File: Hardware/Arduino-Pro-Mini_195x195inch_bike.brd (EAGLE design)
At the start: 49.5 x 49.5 mm, 31 parts, among them Q1 8/16/20MHz, U1 ATMEGA328, U2 MIC5205

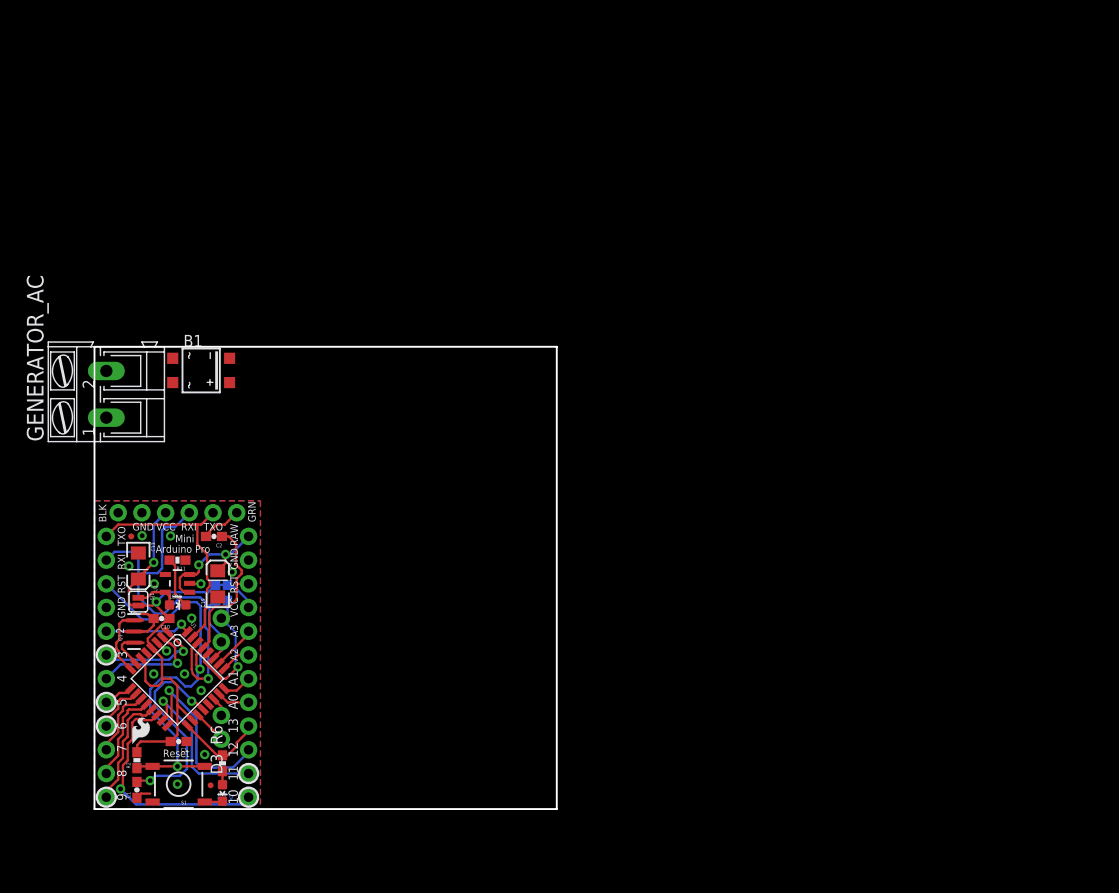
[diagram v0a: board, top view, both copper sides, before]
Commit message: work update, bike draft
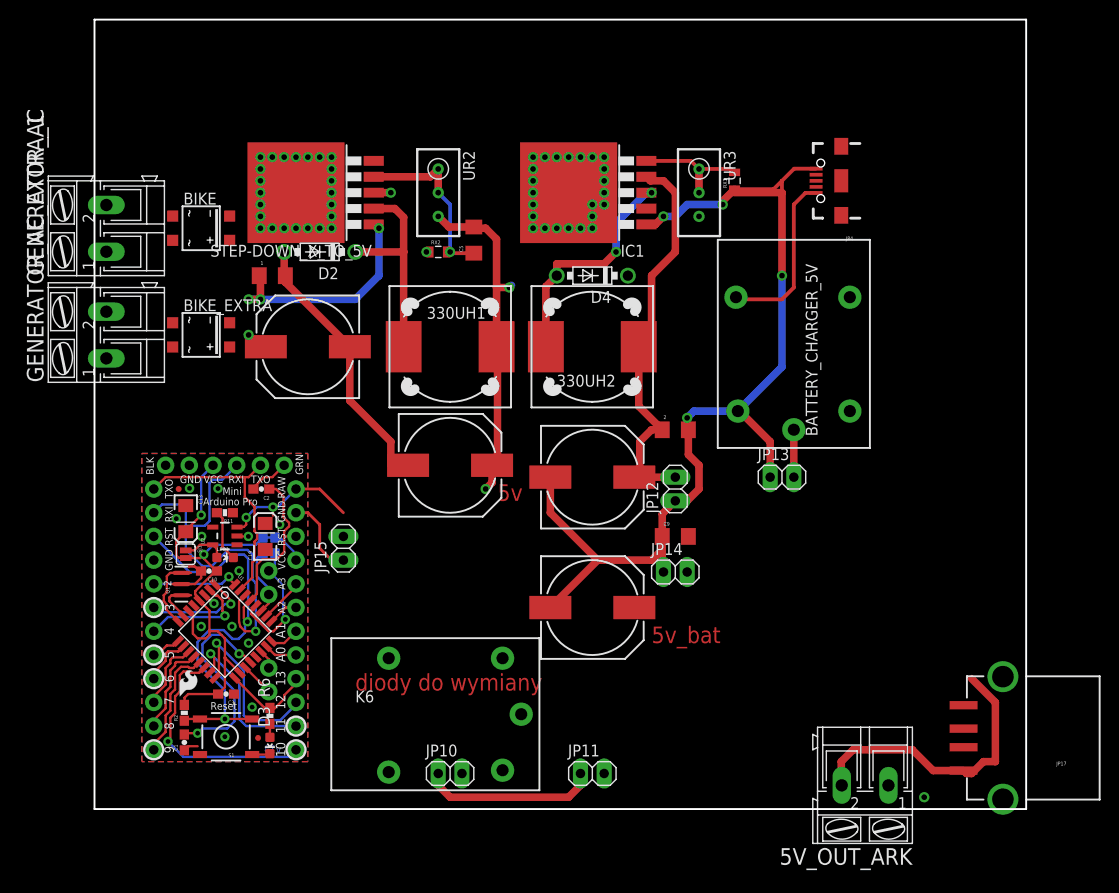
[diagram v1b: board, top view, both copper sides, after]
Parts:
- removed B1: MB1S, rectifier:SOIC-4
- added 1, 2, C5, C9: 100nF, SparkFun-Capacitors:1206
- added 330UH1, 330UH2: DR125, inductors:DR125
- added 5V_OUT_ARK, GENERATOR_AC_EXTRA_1: (no value), con-ptr500:AK300/2
- added BATTERY_CHARGER_5V, K6: ZNS5106, relay:ZN5
- added BIKE, BIKE_EXTRA: MB1S, rectifier:SOIC-4
- added C4, C6, C7, C8: 220uF, SparkFun-Capacitors:NIC_10X10.5_CAP
- added D2, D4: 1N5819-B, diode:DO41-7.6
- added IC1: XL6009_FROM_LM2596S, xl6009:TO263-5
- added JP10, JP11, JP12, JP13, JP14, JP15: (no value), pinhead:1X02
- added JP17: USB_, SparkFun-Connectors:USB-A-S-SILK-FEMALE
- added JP4: USB_MICROB_PLUGCONN-11752, SparkFun-Connectors:USB-B-MICRO-SMD_V03
- added RX2, RX3: 330R, SparkFun-Passives:0805
- added STEP-DOWN_X_TO_5V: LM2596S, national-semiconductor:TO263-5
- added UR2, UR3: 10k, rcl:RTRIM3296W
- moved GENERATOR_AC 17.8 mm to (1.27, 62.2)
- moved C19 7.18 mm to (18.3, 29.2)
- moved LED1 7.18 mm to (14.0, 26.9)
- moved Q1 7.18 mm to (9.32, 24.1)
- moved R1 7.18 mm to (18.1, 28.2)
- moved R3 7.18 mm to (19.3, 28.2)
- moved U$3 7.18 mm to (17.7, 31.5)
- moved C1 7.18 mm to (9.63, 7.14)
- moved C3 7.18 mm to (14.1, 12.3)
- moved D3 7.18 mm to (18.8, 6.81)
- moved JP3 7.18 mm to (18.7, 12.6)
- moved JP7 7.18 mm to (6.35, 6.35)
- moved JP8 7.18 mm to (17.5, 7.62)
- moved R2 7.18 mm to (9.63, 10.3)
- moved R6 7.18 mm to (18.8, 9.98)
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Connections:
- new net 3-4V_LI-ION: 2.1, 330UH2.1, C7.+, IC1.4, JP12.2
- new net 5V: 330UH1.2, BATTERY_CHARGER_5V.12, C5.2, C6.+, JP10.2, JP4.VBUS1, K6.14, UR2.3
- new net 5V_FROM_BATTERY: C19.A, C8.+, C9.2, D4.C, JP14.2, JP15.2, K6.12, U2.1, U2.3, UR3.3
- new net BIKE: BIKE.~2, GENERATOR_AC.1
- new net BIKE+: 1.1, BIKE.+, BIKE_EXTRA.+, C4.+, STEP-DOWN_X_TO_5V.1
- new net N$15: C5.1, RX2.2, STEP-DOWN_X_TO_5V.4, UR2.1, UR2.2
- new net N$16: BATTERY_CHARGER_5V.11, JP13.2
- new net N$17: 330UH1.1, D2.C, STEP-DOWN_X_TO_5V.2
- new net N$19: IC1.5, RX3.2, UR3.1, UR3.2
- new net N$21: 5V_OUT_ARK.2, JP11.2, JP17.VBUS, K6.11
- new net N$25: K6.A1
- new net N$26: BATTERY_CHARGER_5V.A1
- new net N$8: BIKE_EXTRA.~2, GENERATOR_AC_EXTRA_1.1
- new net N$9: BIKE_EXTRA.~1, GENERATOR_AC_EXTRA_1.2
- net GND: now also 1.2, 2.2, 5V_OUT_ARK.1, BATTERY_CHARGER_5V.A2, BIKE.-, BIKE_EXTRA.-, C4.-, C6.-, C7.-, C8.-, C9.1, D2.A, IC1.1, JP10.1, JP11.1, JP12.1, JP13.1, JP14.1, JP15.1, JP17.GND, JP4.GND1, K6.A2, RX2.1, RX3.1, STEP-DOWN_X_TO_5V.3, STEP-DOWN_X_TO_5V.5
- net N$5: now also 330UH2.2, D4.A, IC1.3; no longer B1.~2, GENERATOR_AC.1
- net N$6: now also BIKE.~1; no longer B1.~1
- net RAW: no longer C19.A, U2.1, U2.3
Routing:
- net GND: track 9.36 -> 179.9 mm, vias 13 -> 17
- net 5V: track 0.00 -> 54.7 mm, vias 0 -> 2
- net 3-4V_LI-ION: track 0.00 -> 43.0 mm
- net N$21: track 0.00 -> 31.1 mm
- net BIKE+: track 0.00 -> 24.7 mm, vias 0 -> 1
- net N$5: track 0.00 -> 23.9 mm, vias 0 -> 1
- net N$17: track 0.00 -> 22.6 mm
- net N$15: track 0.00 -> 19.6 mm
- net N$19: track 0.00 -> 12.5 mm
- net N$16: track 0.00 -> 5.08 mm
- net RAW: track 14.1 -> 15.5 mm
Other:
- board size 49.5 x 49.5 mm -> 99.8 x 84.6 mm
- board text added: "5v"
- board text added: "5v_bat"
- board text added: "diody do wymiany"
